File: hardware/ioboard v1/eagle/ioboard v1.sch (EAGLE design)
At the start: 5 parts, among them IC1 MCP23017SO, K1 61300611021, K2 613006143121, K3 691402910008, K4 691402910008

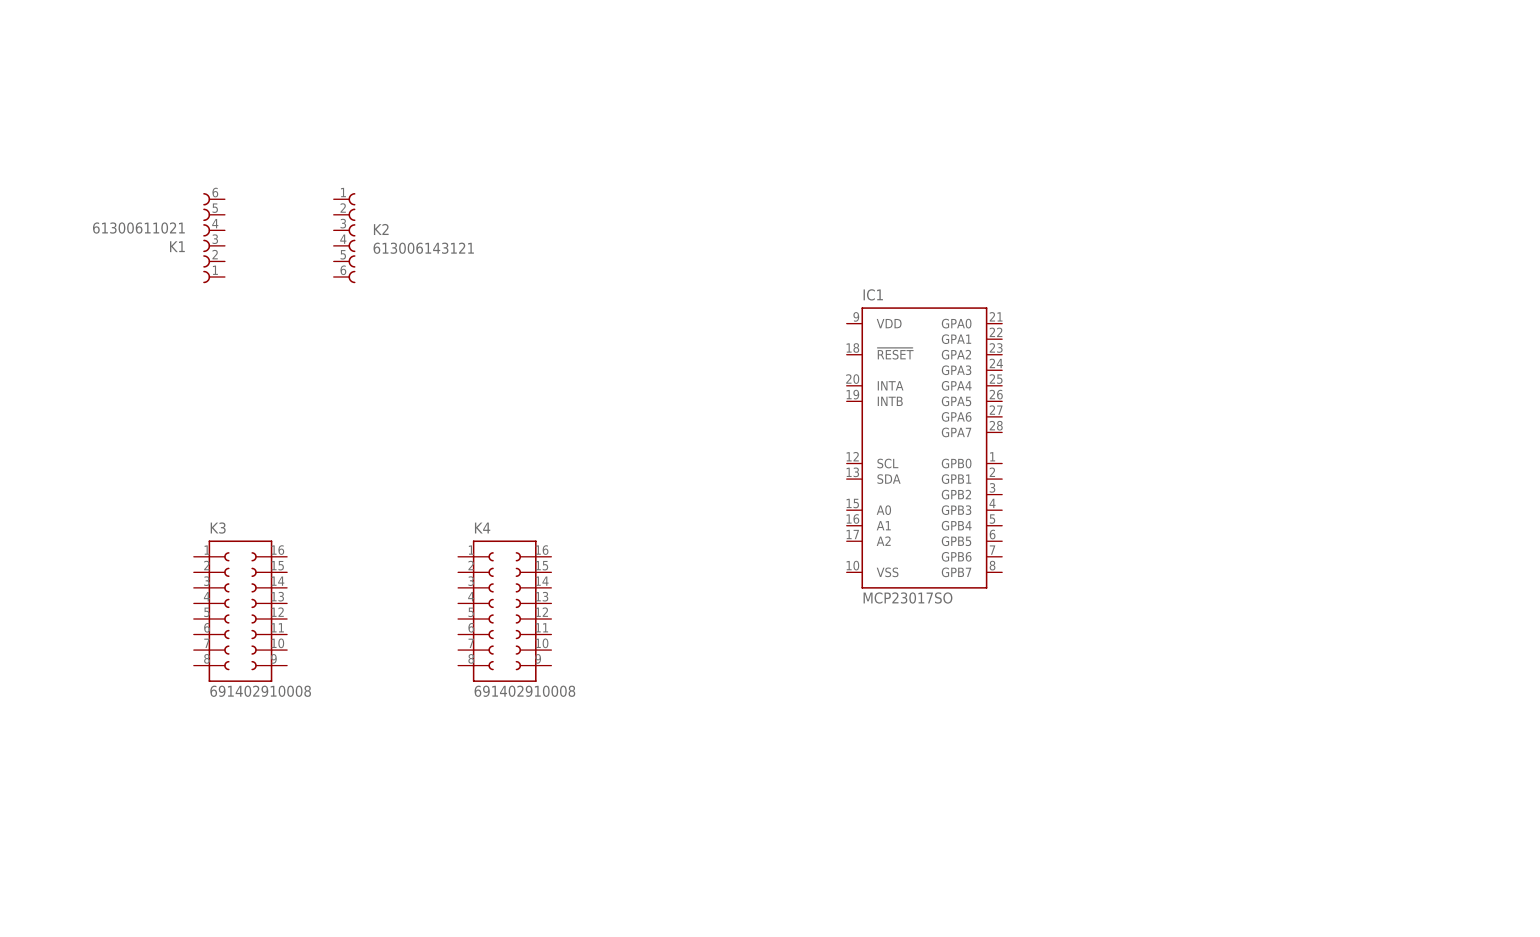
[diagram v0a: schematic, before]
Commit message: Intermediate commit of ioboard.
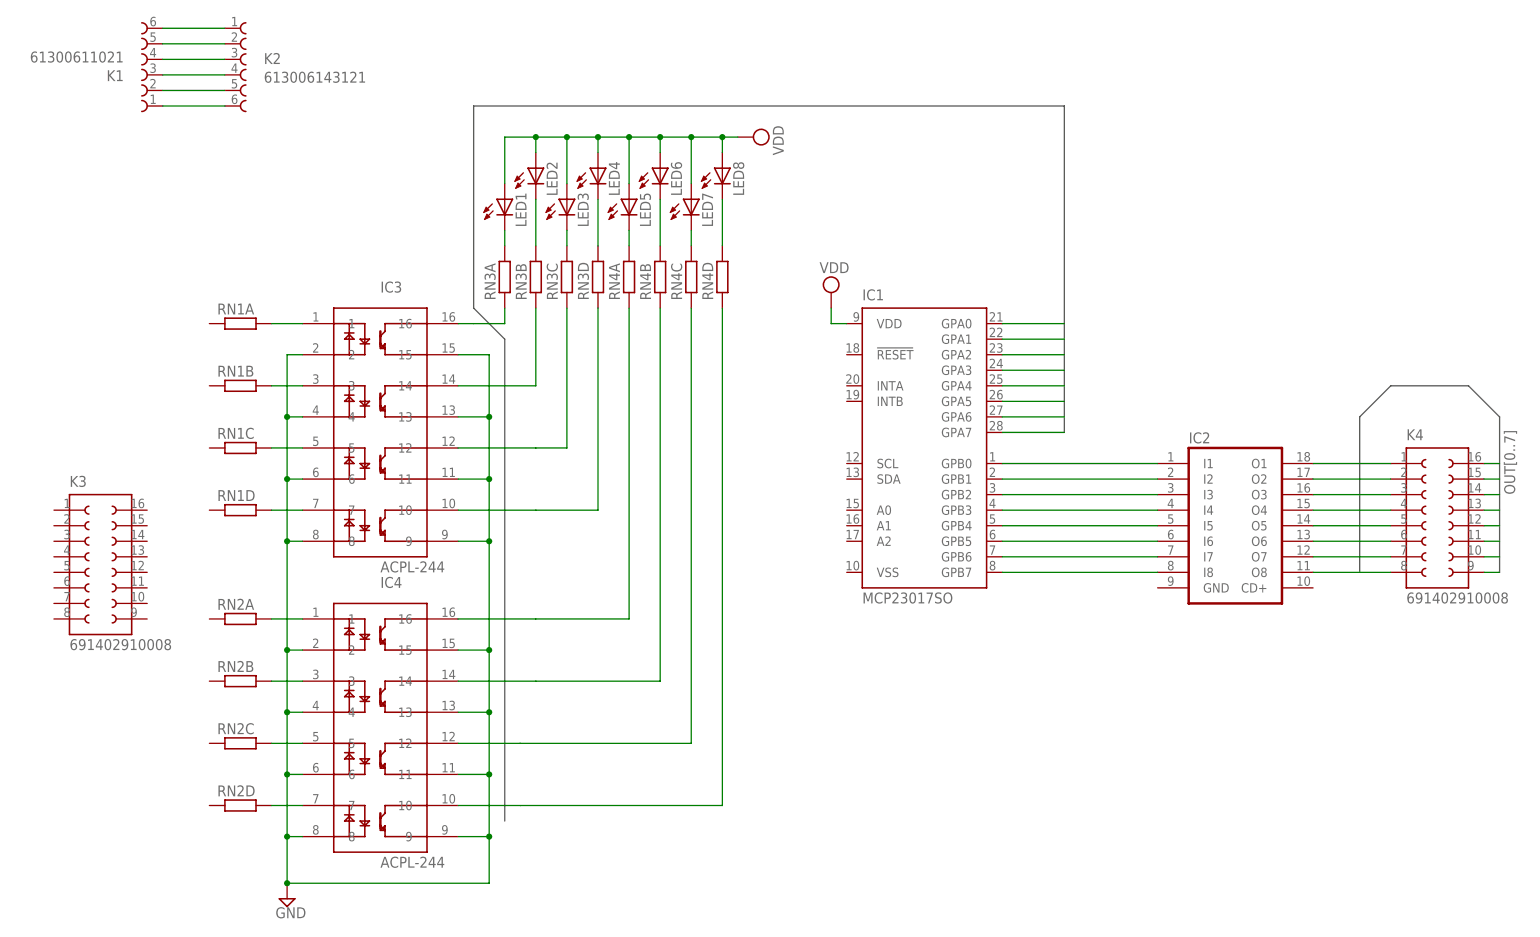
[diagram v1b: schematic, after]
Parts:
- added IC2: (no value), ic:ULN2803A
- added IC3, IC4: ACPL-244, ic:ACPL-244
- added LED1, LED2, LED3, LED4, LED5, LED6, LED7, LED8: (no value), led:LEDCHIPLED_1206
- added RN1, RN2, RN3, RN4: (no value), dp_devices:RESISTOR_ARRAY_4
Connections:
- new net GND: IC3.11, IC3.13, IC3.15, IC3.2, IC3.4, IC3.6, IC3.8, IC3.9, IC4.11, IC4.13, IC4.15, IC4.2, IC4.4, IC4.6, IC4.8, IC4.9
- new net IN_SHIELD0: IC1.GPA0, IC3.16, RN3A.1
- new net IN_SHIELD1: IC1.GPA1, IC3.14, RN3B.1
- new net IN_SHIELD2: IC1.GPA2, IC3.12, RN3C.1
- new net IN_SHIELD3: IC1.GPA3, IC3.10, RN3D.1
- new net IN_SHIELD4: IC1.GPA4, IC4.16, RN4A.1
- new net IN_SHIELD5: IC1.GPA5, IC4.14, RN4B.1
- new net IN_SHIELD6: IC1.GPA6, IC4.12, RN4C.1
- new net IN_SHIELD7: IC1.GPA7, IC4.10, RN4D.1
- new net N$1: IC1.GPB0, IC2.I1
- new net N$10: IC3.3, RN1B.2
- new net N$11: IC3.5, RN1C.2
- new net N$12: IC3.7, RN1D.2
- new net N$13: IC4.1, RN2A.2
- new net N$14: IC4.3, RN2B.2
- new net N$15: IC4.5, RN2C.2
- new net N$16: IC4.7, RN2D.2
- new net N$17: LED1.C, RN3A.2
- new net N$18: LED2.C, RN3B.2
- new net N$19: K1.6, K2.1
- new net N$2: IC1.GPB1, IC2.I2
- new net N$20: K1.5, K2.2
- new net N$21: K1.4, K2.3
- new net N$22: K1.3, K2.4
- new net N$23: K1.2, K2.5
- new net N$24: K1.1, K2.6
- new net N$29: LED3.C, RN3C.2
- new net N$3: IC1.GPB2, IC2.I3
- new net N$30: LED4.C, RN3D.2
- new net N$36: LED5.C, RN4A.2
- new net N$37: LED6.C, RN4B.2
- new net N$38: LED7.C, RN4C.2
- new net N$39: LED8.C, RN4D.2
- new net N$4: IC1.GPB3, IC2.I4
- new net N$5: IC1.GPB4, IC2.I5
- new net N$6: IC1.GPB5, IC2.I6
- new net N$7: IC1.GPB6, IC2.I7
- new net N$8: IC1.GPB7, IC2.I8
- new net N$9: IC3.1, RN1A.2
- new net OUT0: IC2.O1, K4.1, K4.16
- new net OUT1: IC2.O2, K4.15, K4.2
- new net OUT2: IC2.O3, K4.14, K4.3
- new net OUT3: IC2.O4, K4.13, K4.4
- new net OUT4: IC2.O5, K4.12, K4.5
- new net OUT5: IC2.O6, K4.11, K4.6
- new net OUT6: IC2.O7, K4.10, K4.7
- new net OUT7: IC2.O8, K4.8, K4.9
- new net VDD: IC1.VDD, LED1.A, LED2.A, LED3.A, LED4.A, LED5.A, LED6.A, LED7.A, LED8.A
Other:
- moved on the sheet: K1, K2, K3, K4
